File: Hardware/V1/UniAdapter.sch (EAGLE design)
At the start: 24 parts, among them IC1 LD1117S33TR, IC2 SN65HVD232D, IC3 STM32F072CBT6, X1 CAN Bus, X2 CAN Bus

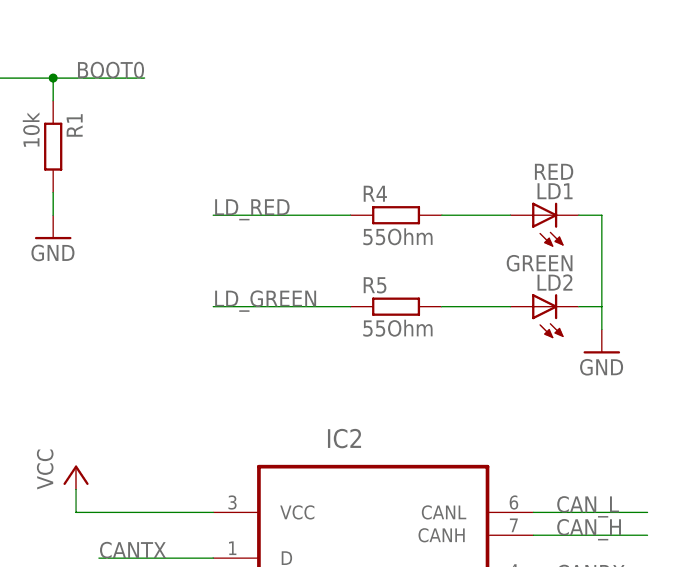
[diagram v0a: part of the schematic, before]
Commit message: AnySense 1.1
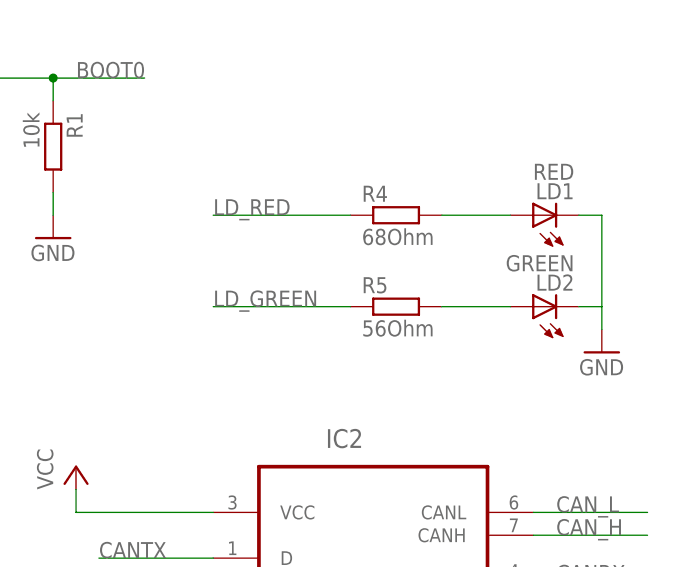
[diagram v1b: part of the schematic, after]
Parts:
- LD1: OC_FARNELL (none) -> 2099221
- LD2: OC_FARNELL (none) -> 2099223
- R4: value 55Ohm -> 68Ohm; OC_FARNELL (none) -> 2331710
- R5: value 55Ohm -> 56Ohm; OC_FARNELL (none) -> 2331709
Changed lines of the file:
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@@
 </part>
 <part name="P+4" library="supply1" deviceset="VCC" device=""/>
-<part name="R4" library="rcl" deviceset="R-EU_" device="R0603" value="55Ohm"/>
-<part name="R5" library="rcl" deviceset="R-EU_" device="R0603" value="55Ohm"/>
-<part name="LD1" library="led" deviceset="LED" device="CHIPLED_0603" value="RED"/>
-<part name="LD2" library="led" deviceset="LED" device="CHIPLED_0603" value="GREEN"/>
+<part name="R4" library="rcl" deviceset="R-EU_" device="R0603" value="68Ohm">
+<attribute name="OC_FARNELL" value="2331710"/>
+</part>
+<part name="R5" library="rcl" deviceset="R-EU_" device="R0603" value="56Ohm">
+<attribute name="OC_FARNELL" value="2331709"/>
+</part>
+<part name="LD1" library="led" deviceset="LED" device="CHIPLED_0603" value="RED">
+<attribute name="OC_FARNELL" value="2099221"/>
+</part>
+<part name="LD2" library="led" deviceset="LED" device="CHIPLED_0603" value="GREEN">
+<attribute name="OC_FARNELL" value="2099223"/>
+</part>
 <part name="GND5" library="supply1" deviceset="GND" device=""/>
 </parts>
@@
 </instance>
 <instance part="P+4" gate="VCC" x="68.58" y="-63.5"/>
-<instance part="R4" gate="G$1" x="111.76" y="30.48"/>
-<instance part="R5" gate="G$1" x="111.76" y="20.32"/>
-<instance part="LD1" gate="G$1" x="127" y="30.48" rot="R90"/>
-<instance part="LD2" gate="G$1" x="127" y="20.32" rot="R90"/>
+<instance part="R4" gate="G$1" x="111.76" y="30.48">
+<attribute name="OC_FARNELL" x="111.76" y="30.48" size="1.778" layer="96" display="off"/>
+</instance>
+<instance part="R5" gate="G$1" x="111.76" y="20.32">
+<attribute name="OC_FARNELL" x="111.76" y="20.32" size="1.778" layer="96" display="off"/>
+</instance>
+<instance part="LD1" gate="G$1" x="127" y="30.48" rot="R90">
+<attribute name="OC_FARNELL" x="127" y="30.48" size="1.778" layer="96" rot="R90" display="off"/>
+</instance>
+<instance part="LD2" gate="G$1" x="127" y="20.32" rot="R90">
+<attribute name="OC_FARNELL" x="127" y="20.32" size="1.778" layer="96" rot="R90" display="off"/>
+</instance>
 <instance part="GND5" gate="1" x="134.62" y="15.24"/>
 </instances>

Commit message: Revert "AnySense 1.1"
This reverts commit 53d5508880b3b2ed964bc1ff9d3bc3f9eadd301f.
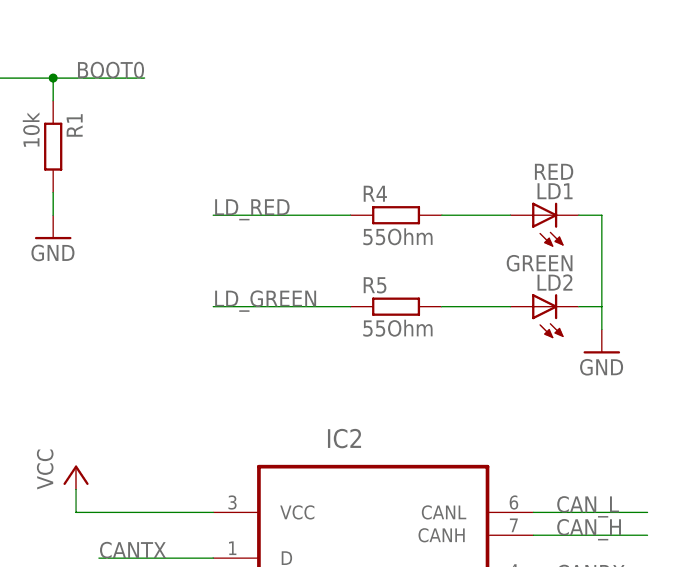
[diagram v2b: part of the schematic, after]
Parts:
- LD1: OC_FARNELL 2099221 -> (none)
- LD2: OC_FARNELL 2099223 -> (none)
- R4: value 68Ohm -> 55Ohm; OC_FARNELL 2331710 -> (none)
- R5: value 56Ohm -> 55Ohm; OC_FARNELL 2331709 -> (none)
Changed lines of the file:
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@@
 </part>
 <part name="P+4" library="supply1" deviceset="VCC" device=""/>
-<part name="R4" library="rcl" deviceset="R-EU_" device="R0603" value="68Ohm">
-<attribute name="OC_FARNELL" value="2331710"/>
-</part>
-<part name="R5" library="rcl" deviceset="R-EU_" device="R0603" value="56Ohm">
-<attribute name="OC_FARNELL" value="2331709"/>
-</part>
-<part name="LD1" library="led" deviceset="LED" device="CHIPLED_0603" value="RED">
-<attribute name="OC_FARNELL" value="2099221"/>
-</part>
-<part name="LD2" library="led" deviceset="LED" device="CHIPLED_0603" value="GREEN">
-<attribute name="OC_FARNELL" value="2099223"/>
-</part>
+<part name="R4" library="rcl" deviceset="R-EU_" device="R0603" value="55Ohm"/>
+<part name="R5" library="rcl" deviceset="R-EU_" device="R0603" value="55Ohm"/>
+<part name="LD1" library="led" deviceset="LED" device="CHIPLED_0603" value="RED"/>
+<part name="LD2" library="led" deviceset="LED" device="CHIPLED_0603" value="GREEN"/>
 <part name="GND5" library="supply1" deviceset="GND" device=""/>
 </parts>
@@
 </instance>
 <instance part="P+4" gate="VCC" x="68.58" y="-63.5"/>
-<instance part="R4" gate="G$1" x="111.76" y="30.48">
-<attribute name="OC_FARNELL" x="111.76" y="30.48" size="1.778" layer="96" display="off"/>
-</instance>
-<instance part="R5" gate="G$1" x="111.76" y="20.32">
-<attribute name="OC_FARNELL" x="111.76" y="20.32" size="1.778" layer="96" display="off"/>
-</instance>
-<instance part="LD1" gate="G$1" x="127" y="30.48" rot="R90">
-<attribute name="OC_FARNELL" x="127" y="30.48" size="1.778" layer="96" rot="R90" display="off"/>
-</instance>
-<instance part="LD2" gate="G$1" x="127" y="20.32" rot="R90">
-<attribute name="OC_FARNELL" x="127" y="20.32" size="1.778" layer="96" rot="R90" display="off"/>
-</instance>
+<instance part="R4" gate="G$1" x="111.76" y="30.48"/>
+<instance part="R5" gate="G$1" x="111.76" y="20.32"/>
+<instance part="LD1" gate="G$1" x="127" y="30.48" rot="R90"/>
+<instance part="LD2" gate="G$1" x="127" y="20.32" rot="R90"/>
 <instance part="GND5" gate="1" x="134.62" y="15.24"/>
 </instances>
